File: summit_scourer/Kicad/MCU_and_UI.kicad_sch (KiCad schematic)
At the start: 5 parts, among them J1 SI5351_breakout_board

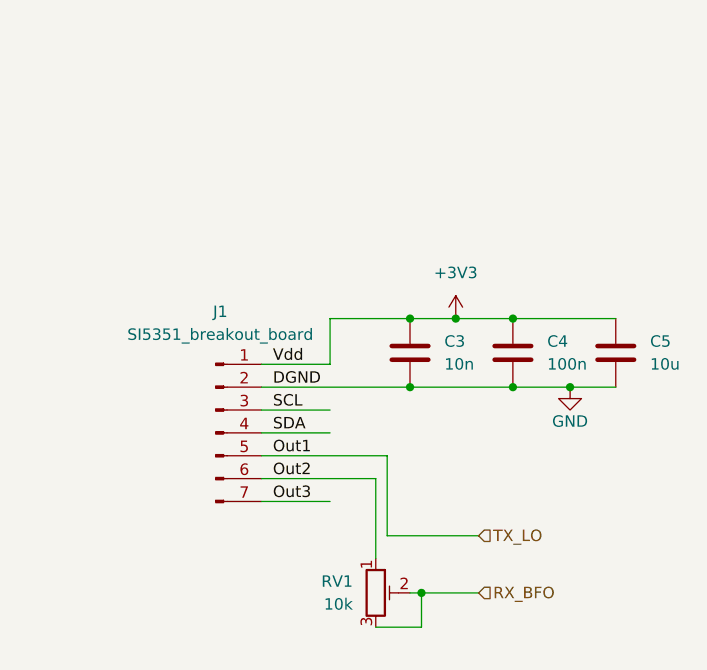
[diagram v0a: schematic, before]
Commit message: Add files via upload
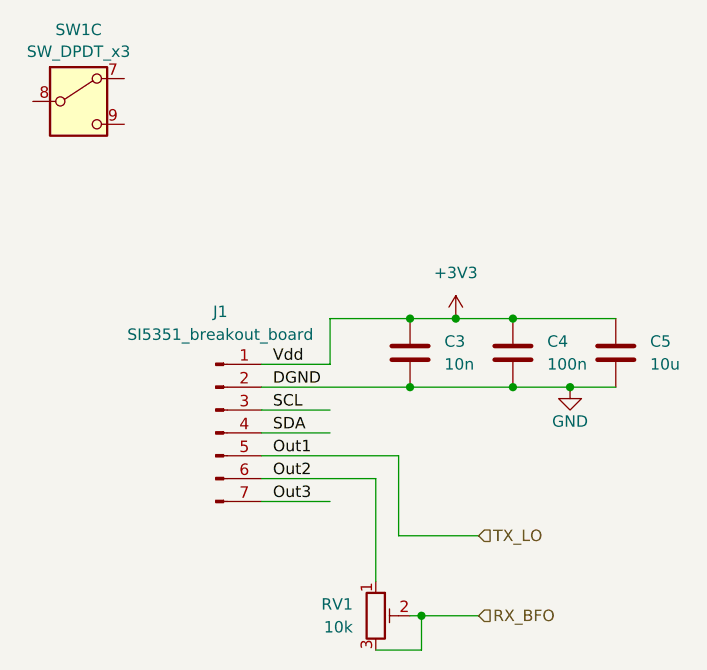
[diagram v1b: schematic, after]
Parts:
- added SW1: SW_DPDT_x3, symbol summit_scourer:SW_DPDT_x3
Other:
- moved on the sheet: RV1
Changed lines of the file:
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@@
 	)
 	(junction
-		(at 208.28 106.68)
+		(at 208.28 109.22)
 		(diameter 0)
 		(color 0 0 0 0)
@@
 	(wire
 		(pts
-			(xy 208.28 106.68) (xy 214.63 106.68)
-		)
-		(stroke
-			(width 0)
-			(type default)
-		)
-	)
-	(wire
-		(pts
-			(xy 204.47 91.44) (xy 204.47 100.33)
+			(xy 208.28 109.22) (xy 214.63 109.22)
+		)
+		(stroke
+			(width 0)
+			(type default)
+		)
+	)
+	(wire
+		(pts
+			(xy 205.74 91.44) (xy 205.74 100.33)
 		)
 		(stroke
@@
 	(wire
 		(pts
-			(xy 208.28 110.49) (xy 208.28 106.68)
+			(xy 208.28 113.03) (xy 208.28 109.22)
 		)
 		(stroke
@@
 	(wire
 		(pts
-			(xy 203.2 93.98) (xy 203.2 102.87)
-		)
-		(stroke
-			(width 0)
-			(type default)
-		)
-	)
-	(wire
-		(pts
-			(xy 203.2 110.49) (xy 208.28 110.49)
-		)
-		(stroke
-			(width 0)
-			(type default)
-		)
-	)
-	(wire
-		(pts
-			(xy 190.5 91.44) (xy 204.47 91.44)
+			(xy 203.2 93.98) (xy 203.2 105.41)
+		)
+		(stroke
+			(width 0)
+			(type default)
+		)
+	)
+	(wire
+		(pts
+			(xy 203.2 113.03) (xy 208.28 113.03)
+		)
+		(stroke
+			(width 0)
+			(type default)
+		)
+	)
+	(wire
+		(pts
+			(xy 190.5 91.44) (xy 205.74 91.44)
 		)
 		(stroke
@@
 	(wire
 		(pts
-			(xy 204.47 100.33) (xy 214.63 100.33)
+			(xy 205.74 100.33) (xy 214.63 100.33)
 		)
 		(stroke
@@
 	(wire
 		(pts
-			(xy 207.01 106.68) (xy 208.28 106.68)
+			(xy 207.01 109.22) (xy 208.28 109.22)
 		)
 		(stroke
@@
 	(hierarchical_label "RX_BFO"
 		(shape input)
-		(at 214.63 106.68 0)
+		(at 214.63 109.22 0)
 		(fields_autoplaced yes)
 		(effects
@@
 					(reference "#PWR03")
 					(unit 1)
+				)
+			)
+		)
+	)
+	(symbol
+		(lib_id "summit_scourer:SW_DPDT_x3")
+		(at 170.18 52.07 0)
+		(unit 3)
+		(exclude_from_sim no)
+		(in_bom yes)
+		(on_board yes)
+		(dnp no)
+		(fields_autoplaced yes)
+		(property "Reference" "SW1"
+			(at 170.18 44.1155 0)
+			(effects
+				(font
+					(size 1.27 1.27)
+				)
+			)
+		)
+		(property "Value" "SW_DPDT_x3"
+			(at 170.18 46.5398 0)
+			(effects
+				(font
+					(size 1.27 1.27)
+				)
+			)
+		)
+		(property "Footprint" ""
+			(at 170.18 52.07 0)
+			(effects
+				(font
+					(size 1.27 1.27)
+				)
+				(hide yes)
+			)
+		)
+		(property "Datasheet" "~"
+			(at 170.18 52.07 0)
+			(effects
+				(font
+					(size 1.27 1.27)
+				)
+				(hide yes)
+			)
+		)
+		(property "Description" "Switch, dual pole double throw, separate symbols"
+			(at 170.18 52.07 0)
+			(effects
+				(font
+					(size 1.27 1.27)
+				)
+				(hide yes)
+			)
+		)
+		(pin "1"
+		)
+		(pin "3"
+		)
+		(pin "8"
+		)
+		(pin "6"
+		)
+		(pin "7"
+		)
+		(pin "9"
+		)
+		(pin "4"
+		)
+		(pin "5"
+		)
+		(pin "2"
+		)
+		(instances
+			(project "summit_scourer"
+				(path "/97fa5a9e-fea2-40ae-976c-23c41ffbf522/9c59661f-2506-4efd-9bc6-e2f1b812693d"
+					(reference "SW1")
+					(unit 3)
 				)
 			)
@@
 	(symbol
 		(lib_id "Device:R_Potentiometer_Trim")
-		(at 203.2 106.68 0)
+		(at 203.2 109.22 0)
 		(unit 1)
 		(exclude_from_sim no)
@@
 		(fields_autoplaced yes)
 		(property "Reference" "RV1"
-			(at 200.66 105.4099 0)
+			(at 200.66 107.9499 0)
 			(effects
 				(font
@@
 		)
 		(property "Value" "10k"
-			(at 200.66 107.9499 0)
+			(at 200.66 110.4899 0)
 			(effects
 				(font
@@
 		)
 		(property "Footprint" ""
-			(at 203.2 106.68 0)
+			(at 203.2 109.22 0)
 			(effects
 				(font
@@
 		)
 		(property "Datasheet" "~"
-			(at 203.2 106.68 0)
+			(at 203.2 109.22 0)
 			(effects
 				(font
@@
 		)
 		(property "Description" "Trim-potentiometer"
-			(at 203.2 106.68 0)
+			(at 203.2 109.22 0)
 			(effects
 				(font
@@
 		)
 		(instances
-			(project ""
+			(project "summit_scourer"
 				(path "/97fa5a9e-fea2-40ae-976c-23c41ffbf522/9c59661f-2506-4efd-9bc6-e2f1b812693d"
 					(reference "RV1")

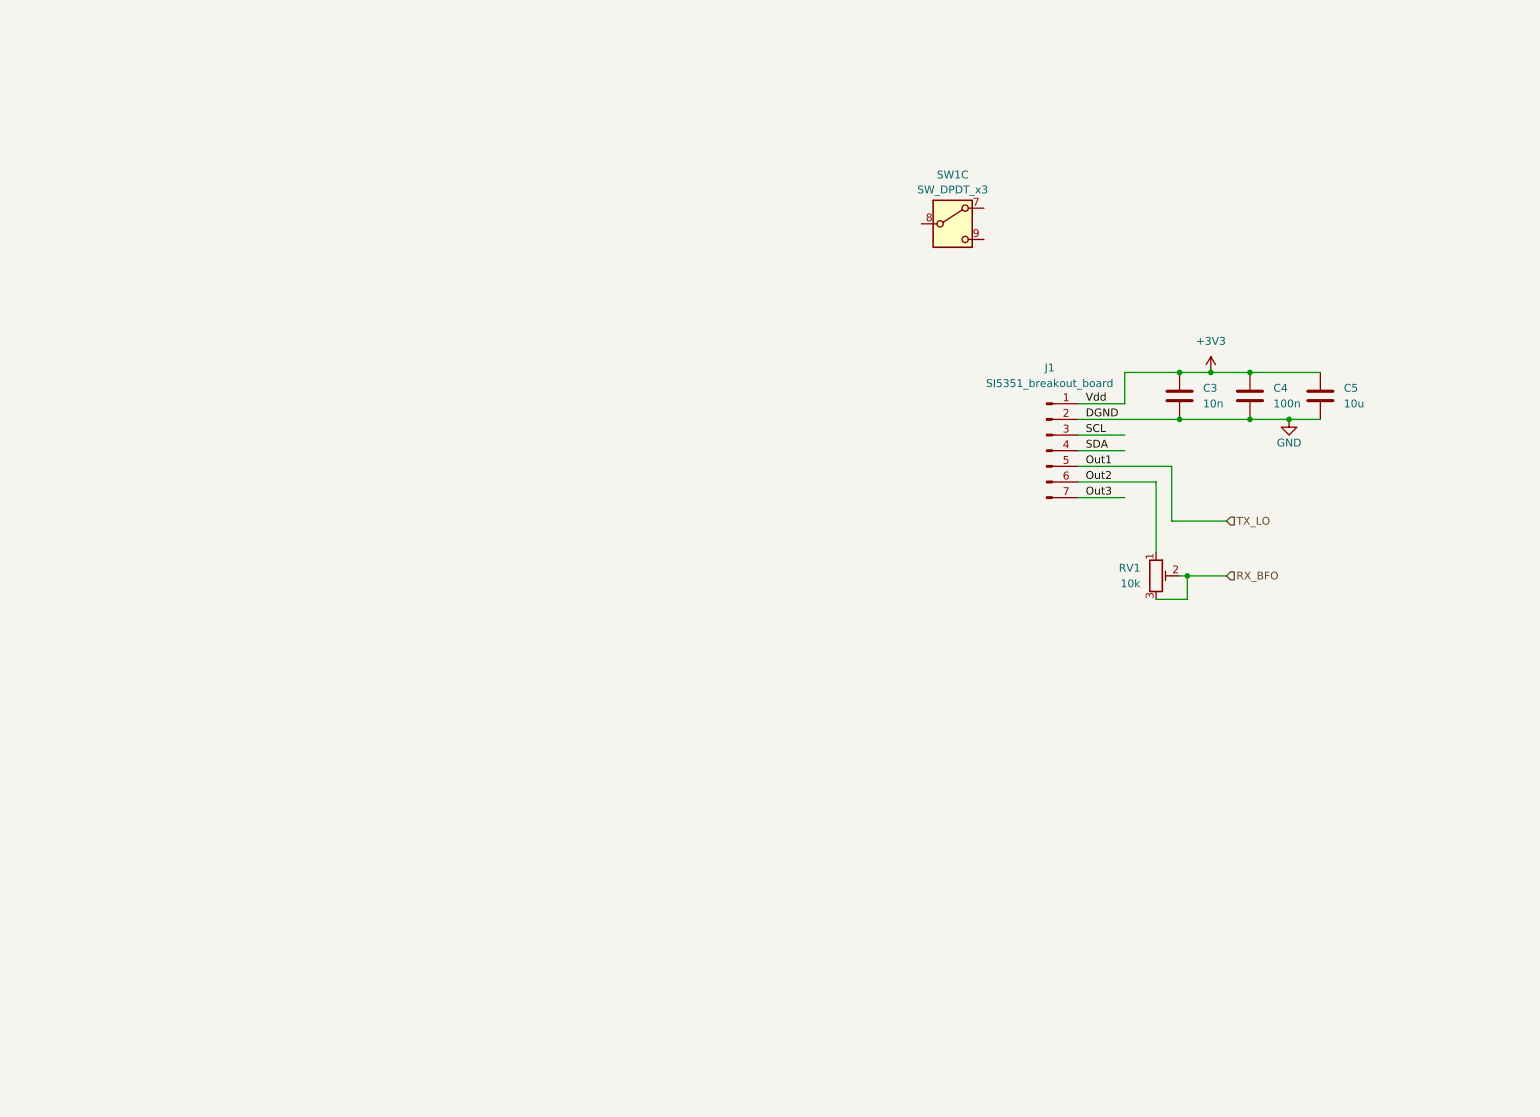
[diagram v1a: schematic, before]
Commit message: Add files via upload
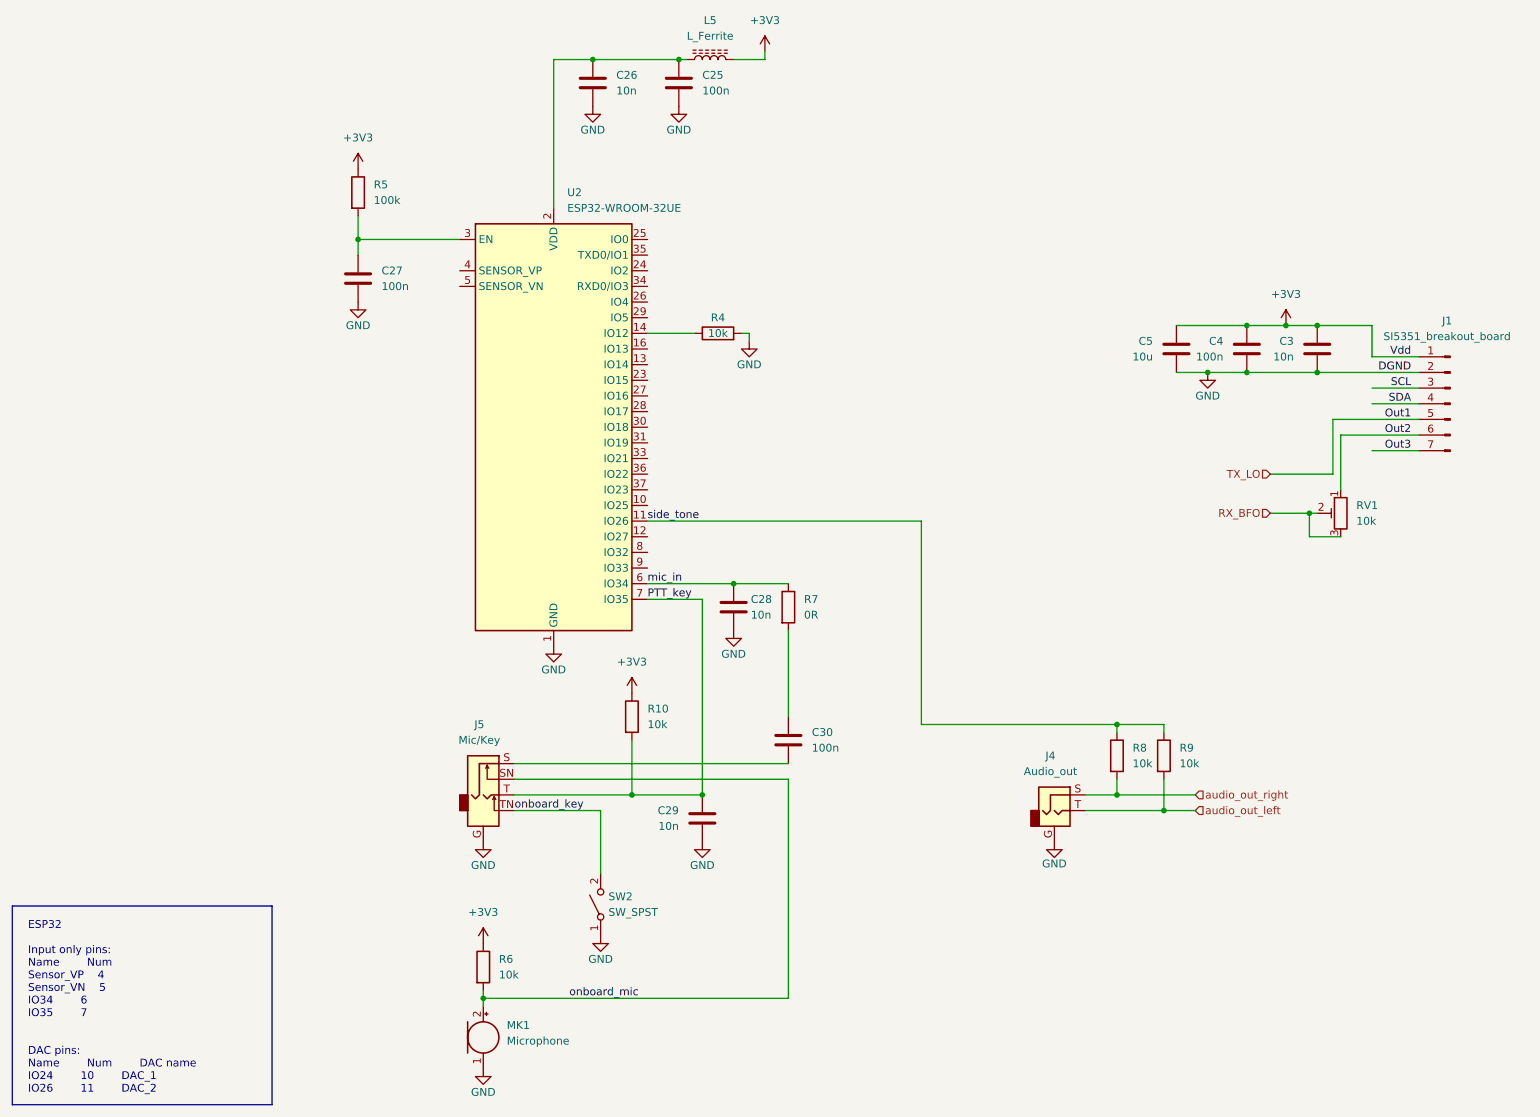
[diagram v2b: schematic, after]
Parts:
- removed SW1: SW_DPDT_x3, symbol summit_scourer:SW_DPDT_x3
- added C25, C27, C30: 100n, Capacitor_SMD:C_0504_1310Metric_Pad0.83x1.28mm_HandSolder, symbol Device:C
- added C26, C28, C29: 10n, Capacitor_SMD:C_0603_1608Metric_Pad1.08x0.95mm_HandSolder, symbol Device:C
- added J4: Audio_out, symbol Connector_Audio:AudioJack2_Ground
- added J5: Mic/Key, symbol Connector_Audio:AudioJack2_Ground_Switch
- added L5: L_Ferrite, symbol Device:L_Ferrite
- added MK1: Microphone, symbol Device:Microphone
- added R10, R4, R6, R8, R9: 10k, symbol Device:R
- added R5: 100k, symbol Device:R
- added R7: 0R, symbol Device:R
- added SW2: SW_SPST, symbol Switch:SW_SPST
- added U2: ESP32-WROOM-32UE, RF_Module:ESP32-WROOM-32UE, symbol RF_Module:ESP32-WROOM-32UE
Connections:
- net +3V3: now also L5.2, R10.1, R5.1, R6.1
- net GND: now also C25.2, C26.2, C27.2, C28.2, C29.2, J4.G, J5.G, MK1.1 (-), R4.2, SW2.1 (A), U2.1 (GND), U2.15 (GND), U2.38 (GND), U2.39 (GND)
- new net: C25.1, C26.1, L5.1, U2.2 (VDD)
- new net: R4.1, U2.14 (IO12)
- new net: C27.1, R5.2, U2.3 (EN)
- new net: C30.1, R7.2
- new net: C30.2, J5.S
- new net PTT_key: C29.1, J5.T, R10.2, U2.7 (IO35)
- new net audio_out_left: J4.T, R9.2
- new net audio_out_right: J4.S, R8.2
- new net mic_in: C28.1, R7.1, U2.6 (IO34)
- new net onboard_key: J5.TN, SW2.2 (B)
- new net onboard_mic: J5.SN, MK1.2 (+), R6.2
- new net side_tone: R8.1, R9.1, U2.11 (IO26)
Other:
- note added: "ESP32 Input only pins: Name Num Sensor_VP 4 Sensor_VN 5 IO34 6 IO35 7 DAC pins: Name Num DAC name IO24 10 DAC_1 IO26 11 DAC_2"
- moved on the sheet: C3, C4, C5, J1, RV1
